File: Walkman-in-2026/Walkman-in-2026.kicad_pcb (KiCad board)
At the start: 2 copper layers, 100 x 63.5 mm, 37 parts, among them J1 AudioJack3, J2 Micro_SD_Card, J3 Conn_01x02_Socket, Q1 BSS138, Q2 BSS138, SW1 SW_Push, SW2 SW_Push, SW3 SW_Push, SW4 SW_SPST, SW5 SW_Push, SW6 SW_Push, U1 XIAO-ESP32-S3-DIP, U2 HS1602A-B, U3 PCM5102, U4 PCF8574P

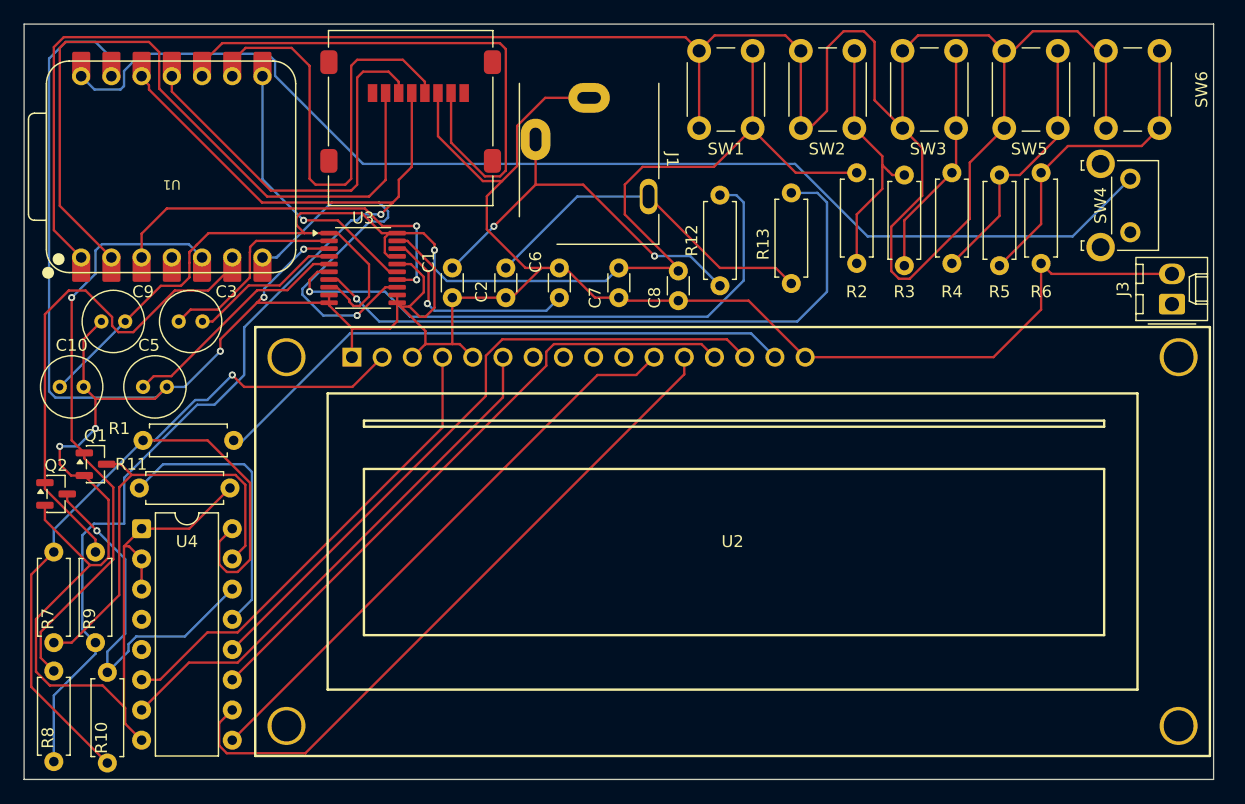
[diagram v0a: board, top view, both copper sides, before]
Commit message: larp
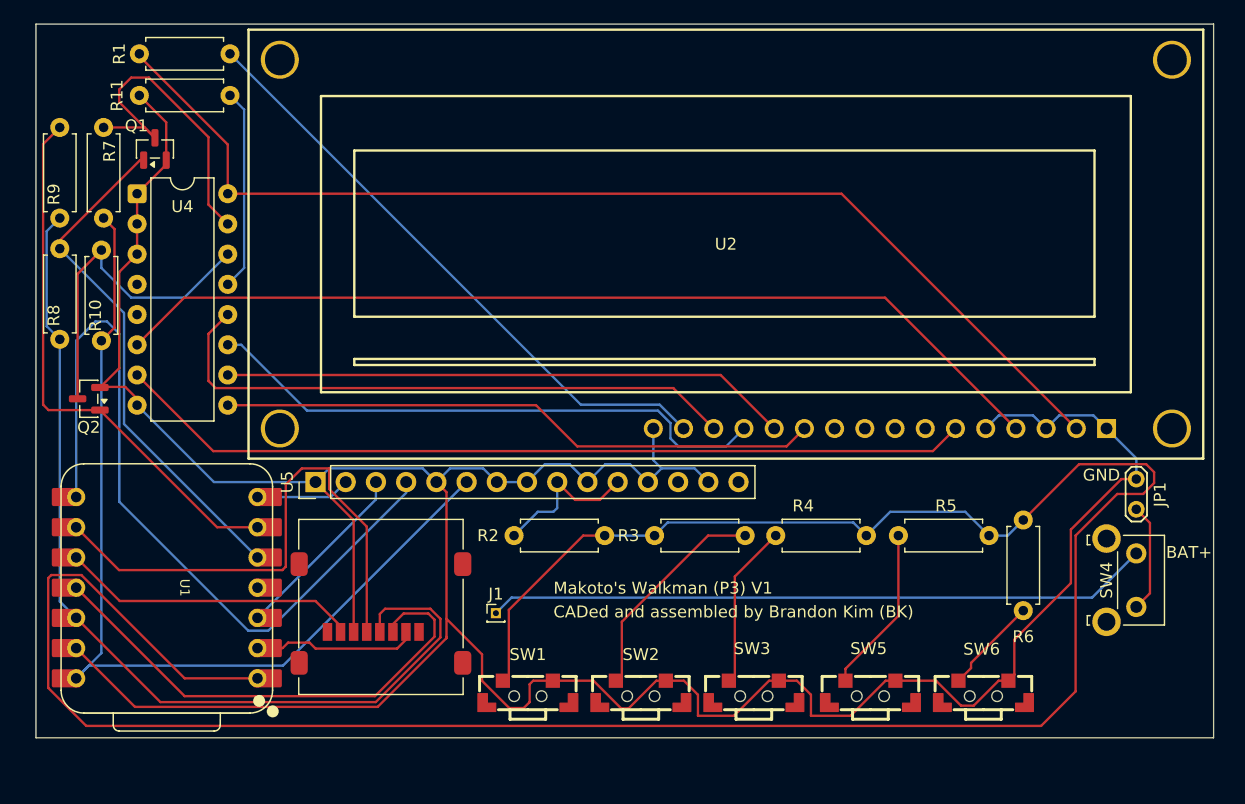
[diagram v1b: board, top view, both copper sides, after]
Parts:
- removed C1, C2: 2.2, Capacitor_THT:C_Disc_D3.0mm_W1.6mm_P2.50mm
- removed C10: 10, Capacitor_THT:C_Radial_D5.0mm_H5.0mm_P2.00mm
- removed C3, C5: 2.2, Capacitor_THT:C_Radial_D5.0mm_H5.0mm_P2.00mm
- removed C6, C7, C8: 0.1, Capacitor_THT:C_Disc_D3.0mm_W1.6mm_P2.50mm
- removed C9: 0.1, Capacitor_THT:C_Radial_D5.0mm_H5.0mm_P2.00mm
- removed J3: Conn_01x02_Socket, Connector_Molex:Molex_KK-254_AE-6410-02A_1x02_P2.54mm_Vertical
- removed R12, R13: 470, Resistor_THT:R_Axial_DIN0207_L6.3mm_D2.5mm_P7.62mm_Horizontal
- removed U3: PCM5102, Package_SO:TSSOP-20_4.4x6.5mm_P0.65mm
- added JP1: Jumper_2_Bridged, TestPoint:TestPoint_2Pads_Pitch2.54mm_Drill0.8mm, F.Cu at (254.5, 111.8)
- added U5: ~, Connector_PinHeader_2.54mm:PinHeader_1x15_P2.54mm_Vertical, F.Cu at (185.5, 112.0)
- J1: value AudioJack3 -> Conn_01x01_Pin; footprint Connector_Audio:Jack_3.5mm_CUI_SJ1-3513N_Horizontal -> Connector_PinHeader_1.00mm:PinHeader_1x01_P1.00mm_Vertical
- R2: value 1k -> 10k
- R4: value 1k -> 4.7k
- R5: value 1k -> 22k
- R6: value 1k -> 47k
- SW1, SW2, SW3, SW5, SW6: footprint Button_Switch_THT:SW_PUSH_6mm -> easyeda2kicad:SW-SMD_TC-S3601-3.5-260G-F0.6
- moved SW1 49.5 mm to (203.3, 129.6), turned to 180 degrees
- moved SW2 49.2 mm to (212.8, 129.6), turned to 180 degrees
- moved SW3 49.0 mm to (222.3, 129.6), turned to 180 degrees
- moved SW5 48.7 mm to (232.2, 129.6), turned to 180 degrees
- moved SW6 48.5 mm to (241.7, 129.6), turned to 180 degrees
- moved J1 44.0 mm to (200.7, 123.0), turned to 0 degrees
- moved R7 43.5 mm to (167.7, 82.2), turned to -90 degrees
- moved J2 41.2 mm to (191.0, 122.5), turned to 180 degrees
- moved R9 35.8 mm to (164.0, 89.8)
- moved R10 35.5 mm to (167.5, 92.5)
- moved R8 35.5 mm to (164.0, 100.0)
- moved U1 35.4 mm to (173.0, 120.9), turned to -90 degrees
- moved R11 33.9 mm to (178.3, 79.5), turned to 180 degrees
- moved R1 32.5 mm to (170.7, 76.0)
- moved SW4 31.5 mm to (254.5, 118.0)
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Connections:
- R10 pad 2: +5V -> VBUS
- R2 pad 1: Net-(R2-Pad1) -> GPIO1
- R3 pad 1: Net-(R3-Pad1) -> GPIO1
- R3 pad 2: Net-(R2-Pad1) -> Net-(R3-Pad2)
- R4 pad 2: Net-(R3-Pad1) -> GPIO1
- R5 pad 1: Net-(R5-Pad1) -> GPIO1
- R5 pad 2: Net-(R4-Pad1) -> Net-(R5-Pad2)
- R6 pad 1: GND -> GPIO1
- R6 pad 2: Net-(R5-Pad1) -> Net-(R6-Pad2)
- R7 pad 2: +5V -> VBUS
- SW1 pad 1: Net-(U1-GPIO1_A0_D0) -> GND
- SW1 pad 2: +3V3 -> GPIO1
- SW2 pad 1: Net-(U1-GPIO1_A0_D0) -> GND
- SW2 pad 2: Net-(R2-Pad1) -> Net-(R3-Pad2)
- SW3 pad 1: Net-(U1-GPIO1_A0_D0) -> GND
- SW3 pad 2: Net-(R3-Pad1) -> Net-(R4-Pad1)
- SW4 pad 1: Net-(SW4-A) -> Net-(J1-Pin_1)
- SW5 pad 1: Net-(U1-GPIO1_A0_D0) -> GND
- SW5 pad 2: Net-(R4-Pad1) -> Net-(R5-Pad2)
- SW6 pad 1: Net-(U1-GPIO1_A0_D0) -> GND
- SW6 pad 2: Net-(R5-Pad1) -> Net-(R6-Pad2)
- U1 pad 1: Net-(U1-GPIO1_A0_D0) -> GPIO1
- U1 pad 14: Net-(SW4-A) -> VBUS
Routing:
- net GPIO1: track 0.00 -> 210.9 mm
- net Net-(U1-GPIO1_A0_D0): track 189.7 -> 0.00 mm
- net +3V3: track 121.1 -> 13.4 mm, vias 1 -> 0
- net Net-(SW4-A): track 99.8 -> 0.00 mm
- net VBUS: track 0.00 -> 80.1 mm
- net Net-(J1-Pin_1): track 0.00 -> 55.9 mm
- net Net-(U3-OUTR): track 55.2 -> 0.00 mm, vias 1 -> 0
- net GND: track 312.0 -> 258.1 mm, vias 5 -> 0
- net Net-(U3-OUTL): track 50.4 -> 0.00 mm, vias 1 -> 0
- net Net-(J2-DAT3/CD): track 62.1 -> 13.9 mm
- net Net-(U1-GPIO44_D7_RX): track 23.2 -> 67.4 mm, vias 1 -> 0
- net Net-(U2-RS): track 40.0 -> 80.1 mm
- net Net-(C1-Pad2): track 32.7 -> 0.00 mm, vias 2 -> 0
- net Net-(C2-Pad2): track 29.5 -> 0.00 mm
- net Net-(U2-E): track 44.6 -> 72.2 mm
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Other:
- board size 100 x 63.5 mm -> 99 x 60 mm
- board text added: "BAT+"
- board text added: "CADed and assembled by Brandon Kim (BK)"
- board text added: "GND"
- board text added: "Makoto's Walkman (P3) V1"
